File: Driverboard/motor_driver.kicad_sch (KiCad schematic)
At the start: 21 parts

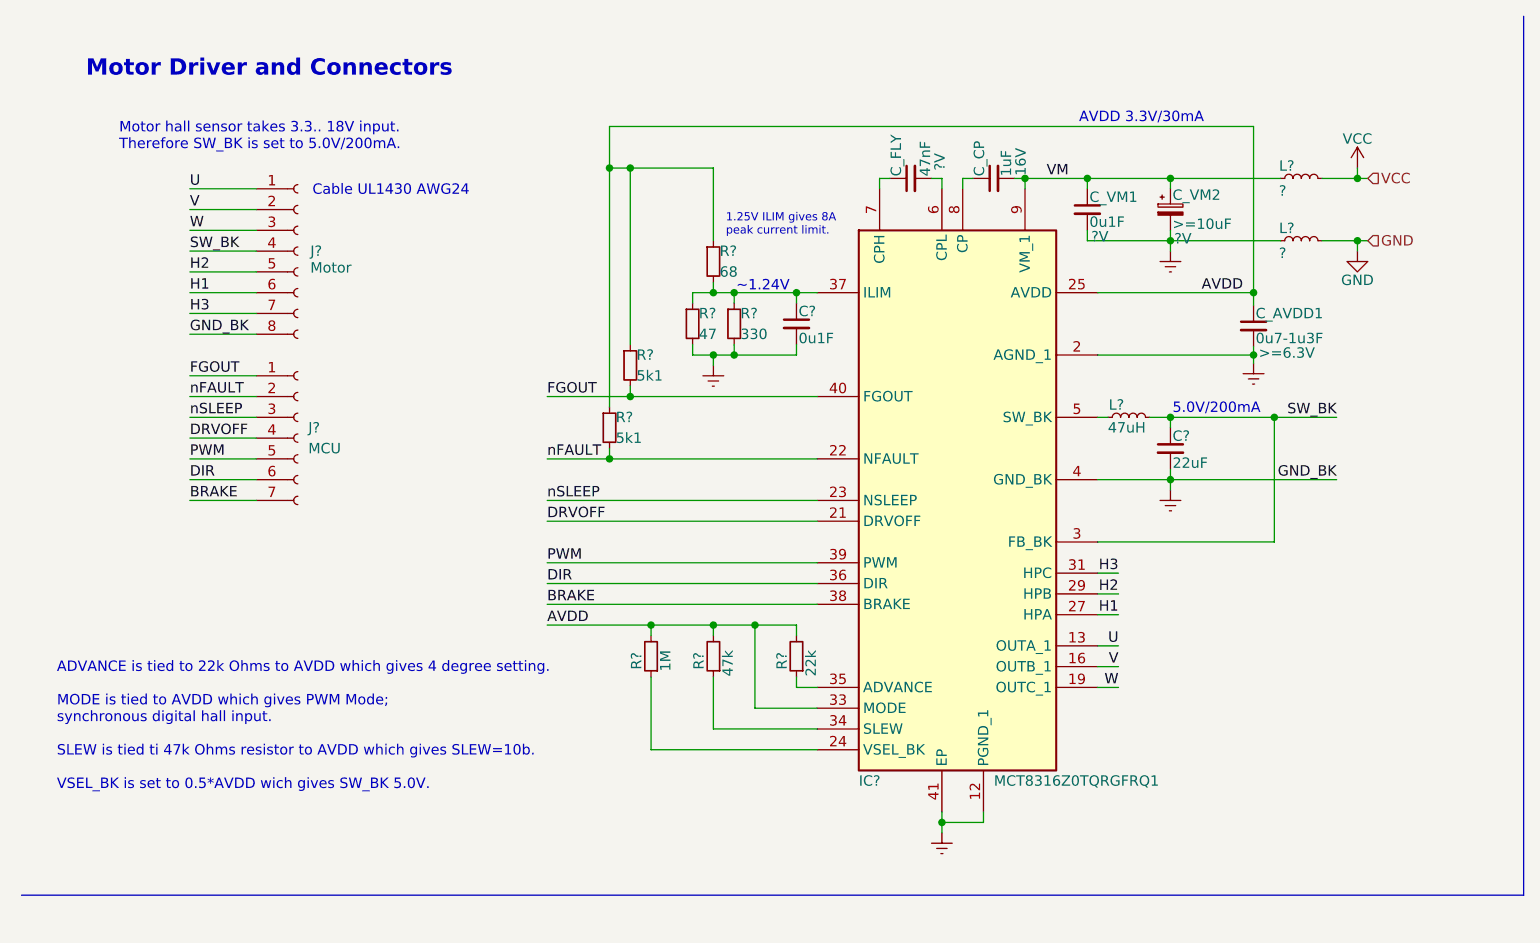
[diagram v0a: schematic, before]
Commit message: WIP
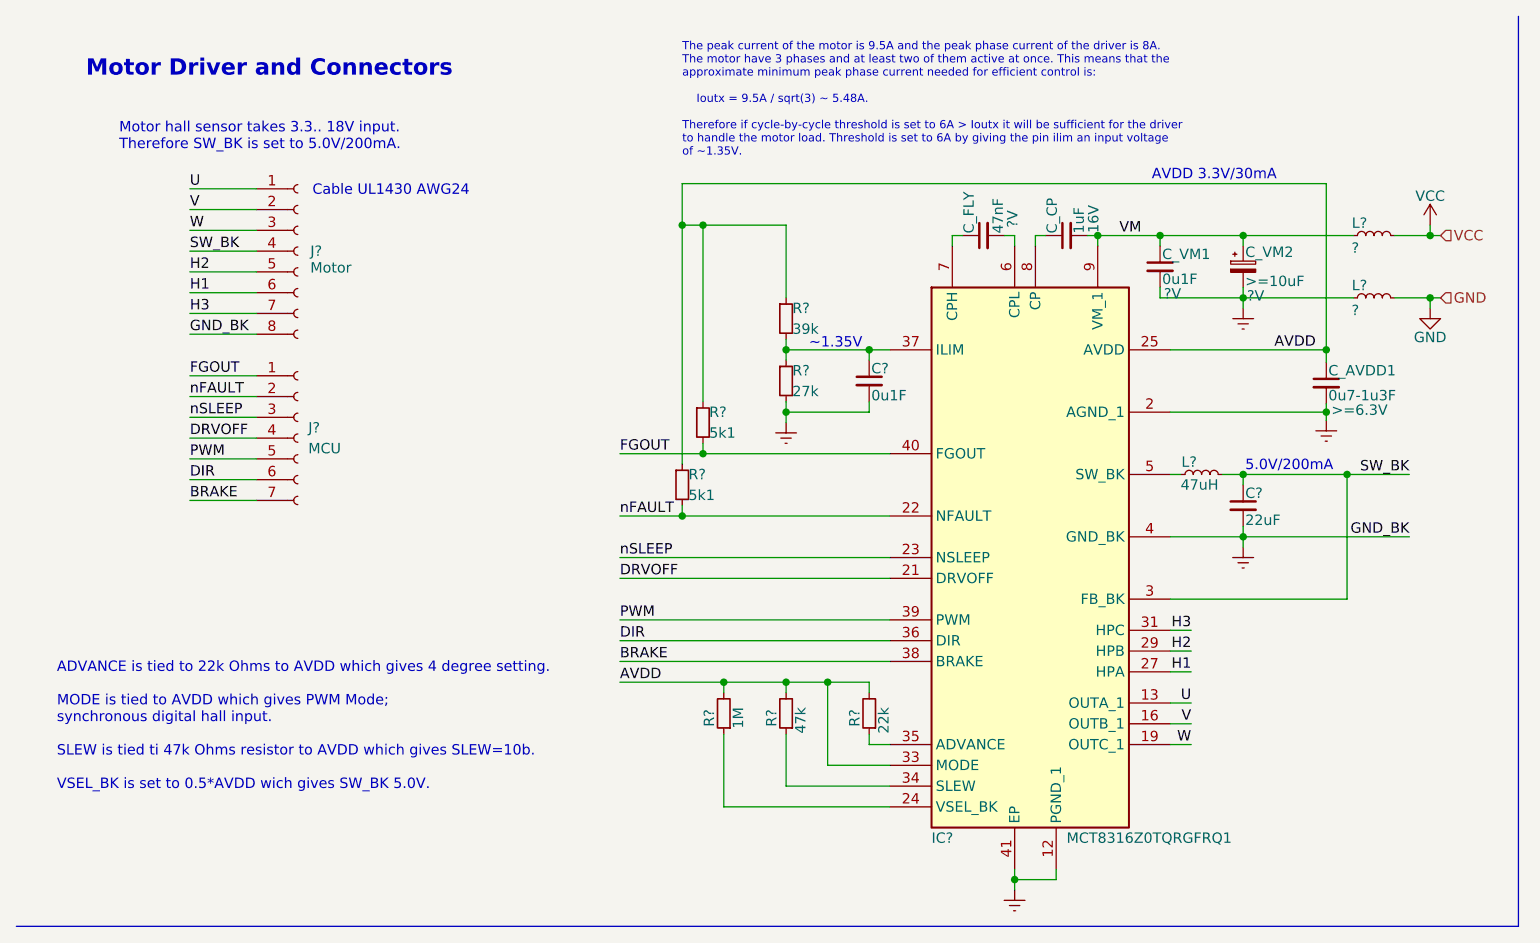
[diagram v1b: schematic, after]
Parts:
- removed R?: 47, symbol Device:R_Small
- R?: value 68 -> 39k
- R?: value 330 -> 27k
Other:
- note added: "The peak current of the motor is 9.5A and the peak phase current of the driver is 8A. The motor have 3 phases and at least two of them active at once. This means that the approximate minimum peak phase current needed for efficient control is: Ioutx = 9.5A / sqrt(3) ~ 5.48A. Therefore if cycle-by-cycle threshold is set to 6A > Ioutx it will be sufficient for the driver to handle the motor load. Th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"
- note added: "~1.35V"
- note removed: "1.25V ILIM gives 8A peak current limit."
- note removed: "~1.24V"
- moved on the sheet: C?, C_AVDD1, C_CP, C_FLY, C_VM1, C_VM2, IC?, L?, R?
